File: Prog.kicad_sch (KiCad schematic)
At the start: 23 parts, among them J2 JTAG, J3 microUSB, Q1 MMBT3904, Q2 MMBT3904, U12 CH340G, U7 74AHCT573PW, Y1 12M

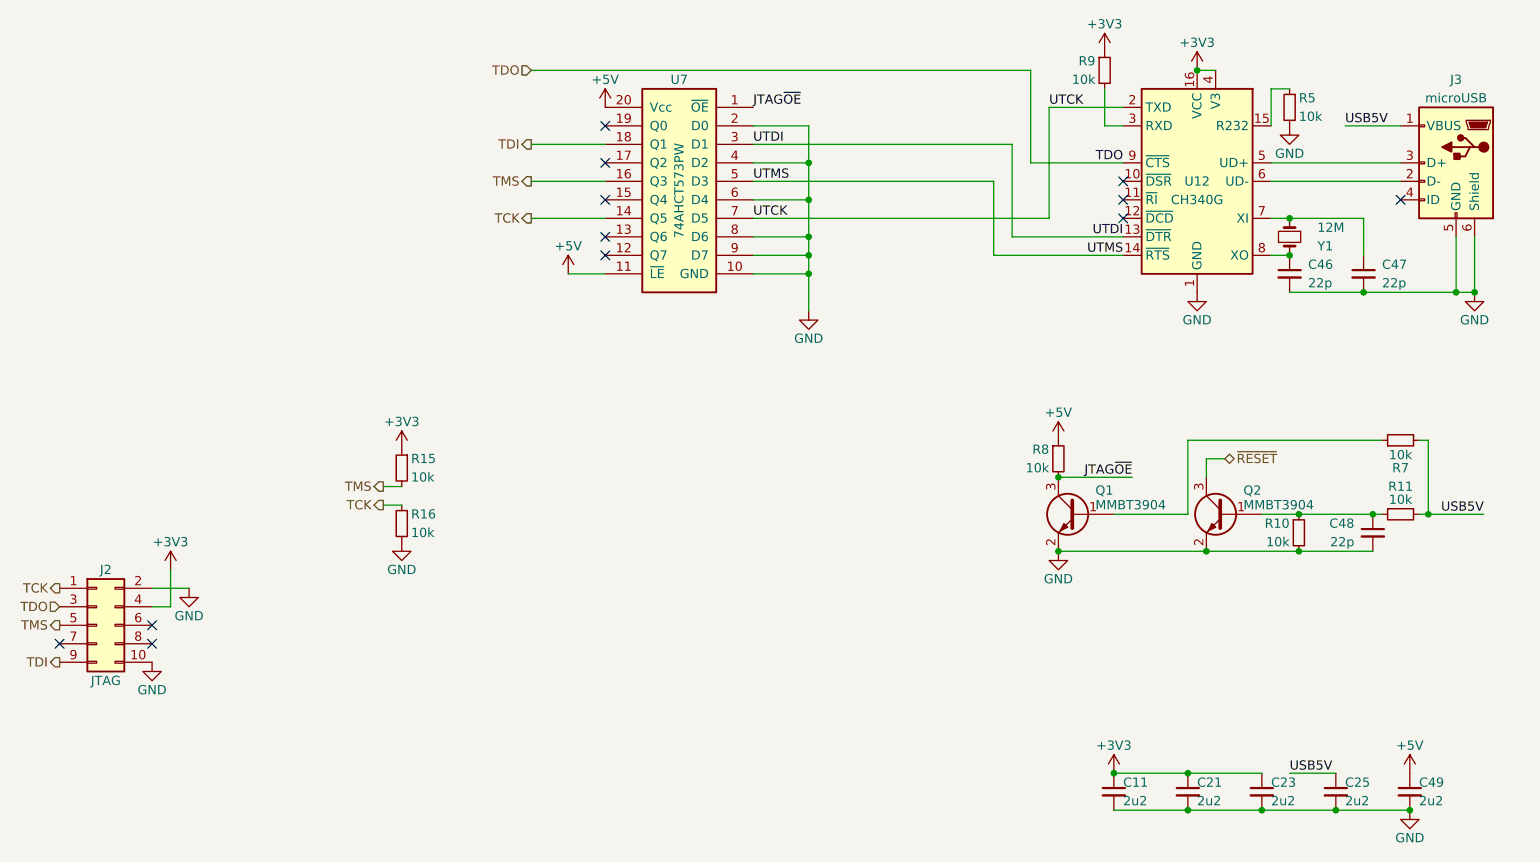
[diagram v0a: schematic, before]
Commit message: idk
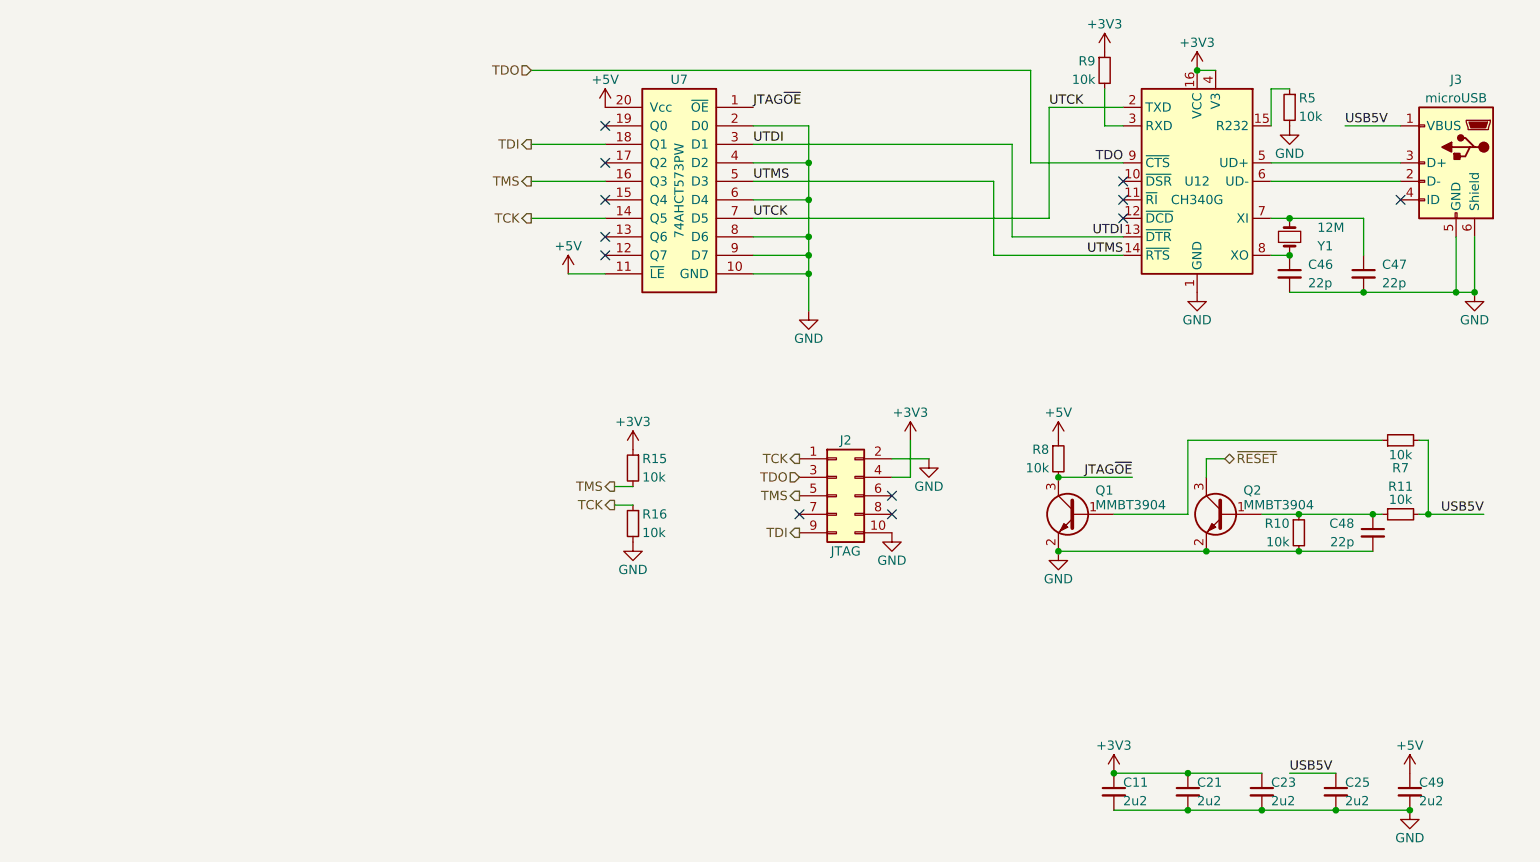
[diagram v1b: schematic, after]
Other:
- moved on the sheet: J2, R15, R16

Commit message: Toward final "A"
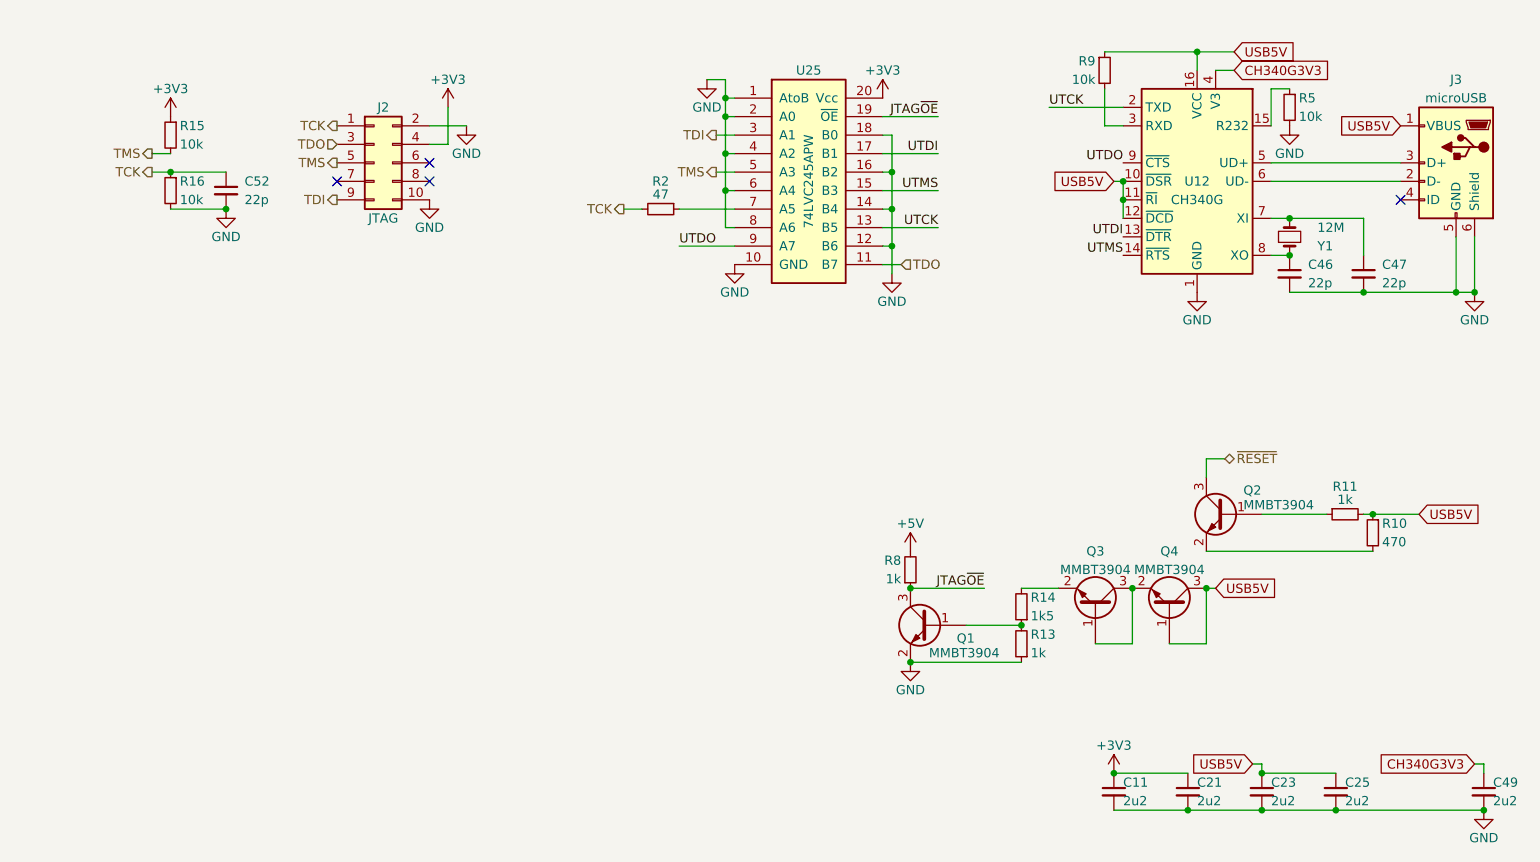
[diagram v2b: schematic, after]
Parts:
- removed C48: 22p, stdpads:C_0603, symbol Device:C_Small
- removed R7: 10k, stdpads:R_0603, symbol Device:R_Small
- removed U7: 74AHCT573PW, stdpads:TSSOP-20_4.4x6.5mm_P0.65mm, symbol GW_Logic:74573
- added C52: 22p, stdpads:C_0603, symbol Device:C_Small
- added Q3, Q4: MMBT3904, stdpads:SOT-23, symbol Transistor_BJT:MMBT3904
- added R13: 1k, stdpads:R_0603, symbol Device:R_Small
- added R14: 1k5, stdpads:R_0603, symbol Device:R_Small
- added R2: 47, stdpads:R_0603, symbol Device:R_Small
- added U25: 74LVC245APW, stdpads:TSSOP-20_4.4x6.5mm_P0.65mm, symbol GW_Logic:74245
- R10: value 10k -> 470; footprint stdpads:R_0603 -> stdpads:R_0805; LCSC Part C25804 -> (none)
- R11, R8: value 10k -> 1k; LCSC Part C25804 -> (none)
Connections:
- net +3V3: now also U25.20 (Vcc); no longer C23.1, R9.1, U12.16 (VCC), U12.4 (V3)
- net +5V: now also R8.2; no longer C49.1, R8.1
- net GND: now also C52.2, R13.1, U25.1 (AtoB), U25.10 (GND), U25.12 (B6), U25.14 (B4), U25.16 (B2), U25.18 (B0), U25.2 (A0), U25.4 (A2), U25.6 (A4), U25.8 (A6); no longer Q2.2 (E), R10.2
- net JTAG~{OE}: now also R8.1, U25.19 (~{OE}); no longer R8.2
- net TCK: now also C52.1, R2.2
- net TDI: now also U25.3 (A1)
- net TDO: now also U25.11 (B7); no longer U12.9 (~{CTS})
- net TMS: now also U25.5 (A3)
- net USB5V: now also C23.1, R10.1, R9.1, U12.10 (~{DSR}), U12.11 (~{RI}), U12.12 (~{DCD}), U12.16 (VCC), Q4.1 (B), Q4.3 (C)
- net UTCK: now also U25.13 (B5)
- net UTDI: now also U25.17 (B1)
- net UTMS: now also U25.15 (B3)
- net at Q2.1 (B), R11.1: no longer R10.1
- net at Q1.1 (B): now also R13.2, R14.1
- new net: Q2.2 (E), R10.2
- new net: R2.1, U25.7 (A5)
- new net: Q3.2 (E), R14.2
- new net: Q3.1 (B), Q3.3 (C), Q4.2 (E)
- new net CH340G3V3: C49.1, U12.4 (V3)
- new net UTDO: U12.9 (~{CTS}), U25.9 (A7)
- no-connect marks 12 -> 4
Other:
- moved on the sheet: C49, J2, Q1, R10, R15, R16

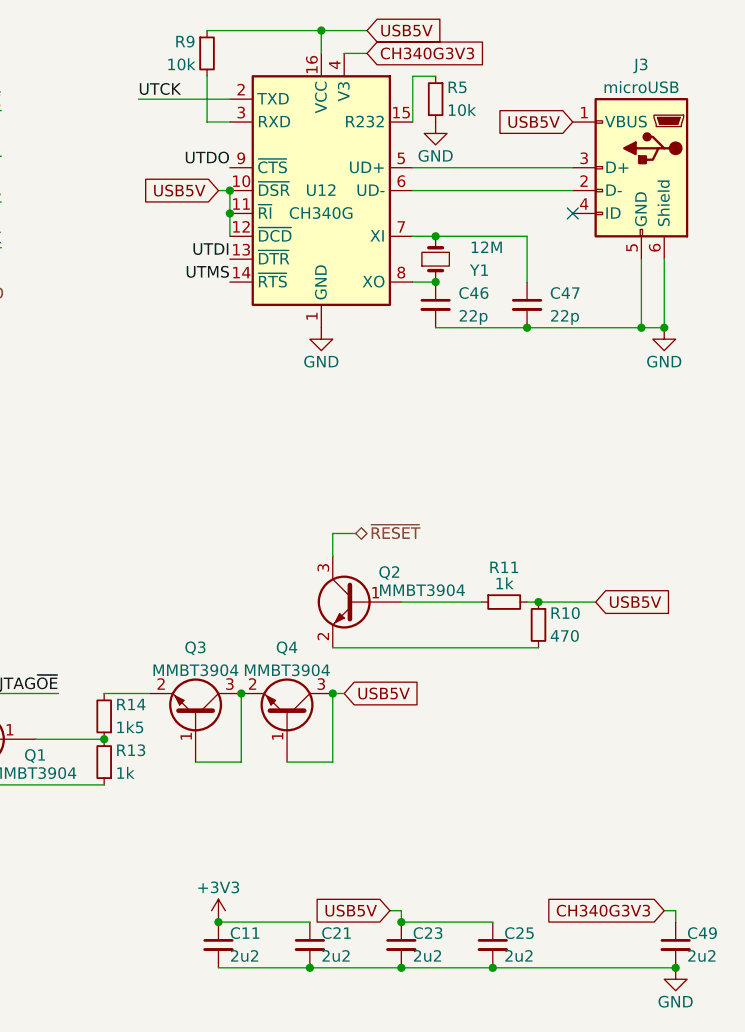
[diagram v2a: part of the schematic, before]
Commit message: idk
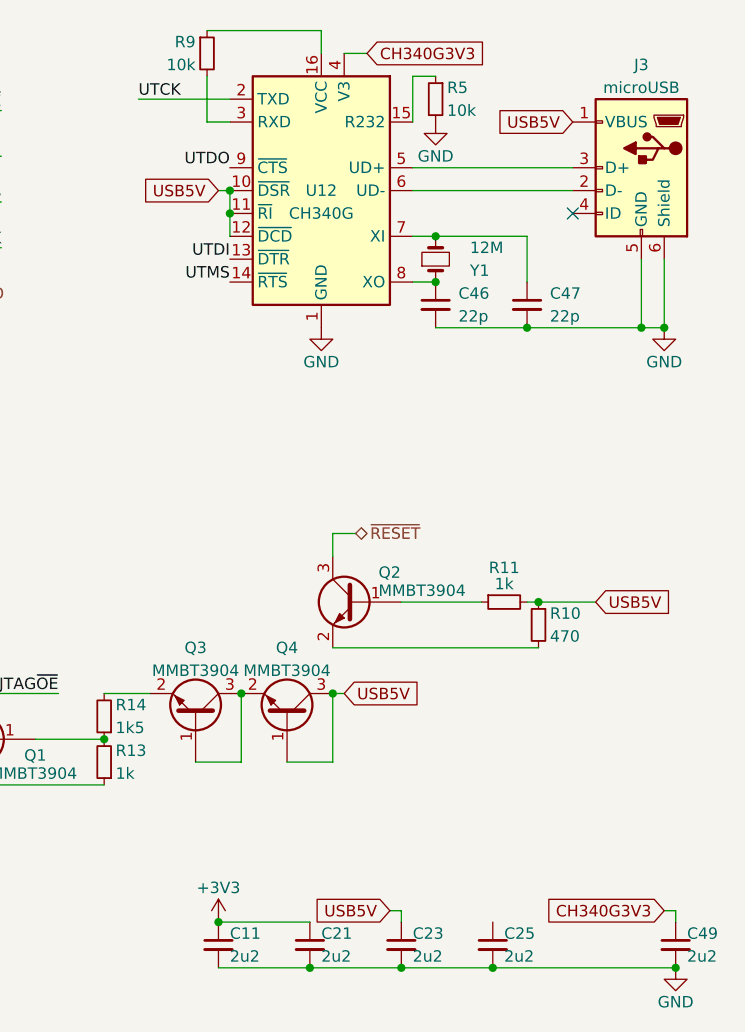
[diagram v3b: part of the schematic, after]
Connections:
- net USB5V: no longer C25.1, R9.1, U12.16 (VCC)
- new net: R9.1, U12.16 (VCC)
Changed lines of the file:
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@@
   (junction (at 156.21 48.26) (diameter 0) (color 0 0 0 0)
   )
-  (junction (at 220.98 41.91) (diameter 0) (color 0 0 0 0)
-  )
   (junction (at 179.07 63.5) (diameter 0) (color 0 0 0 0)
   )
@@
   )
   (junction (at 260.35 146.05) (diameter 0) (color 0 0 0 0)
-  )
-  (junction (at 229.87 140.97) (diameter 0) (color 0 0 0 0)
   )
   (junction (at 219.71 146.05) (diameter 0) (color 0 0 0 0)
@@
     (stroke (width 0) (type default))
   )
-  (wire (pts (xy 229.87 140.97) (xy 240.03 140.97))
-    (stroke (width 0) (type default))
-  )
   (wire (pts (xy 208.28 46.99) (xy 208.28 52.07))
     (stroke (width 0) (type default))
@@
   )
   (wire (pts (xy 224.79 97.79) (xy 222.25 97.79))
-    (stroke (width 0) (type default))
-  )
-  (wire (pts (xy 220.98 41.91) (xy 226.06 41.91))
     (stroke (width 0) (type default))
   )
@@
     )
   )
-  (global_label "USB5V" (shape input) (at 226.06 41.91 0) (fields_autoplaced)
-    (effects (font (size 1.27 1.27)) (justify left))
-    (property "Intersheetrefs" "${INTERSHEET_REFS}" (at 234.4197 41.91 0)
-      (effects (font (size 1.27 1.27)) (justify left) hide)
-    )
-  )

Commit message: Revert "idk"
This reverts commit aa30aa8a559ae1d3e965923a55380a6d00f93ea4.
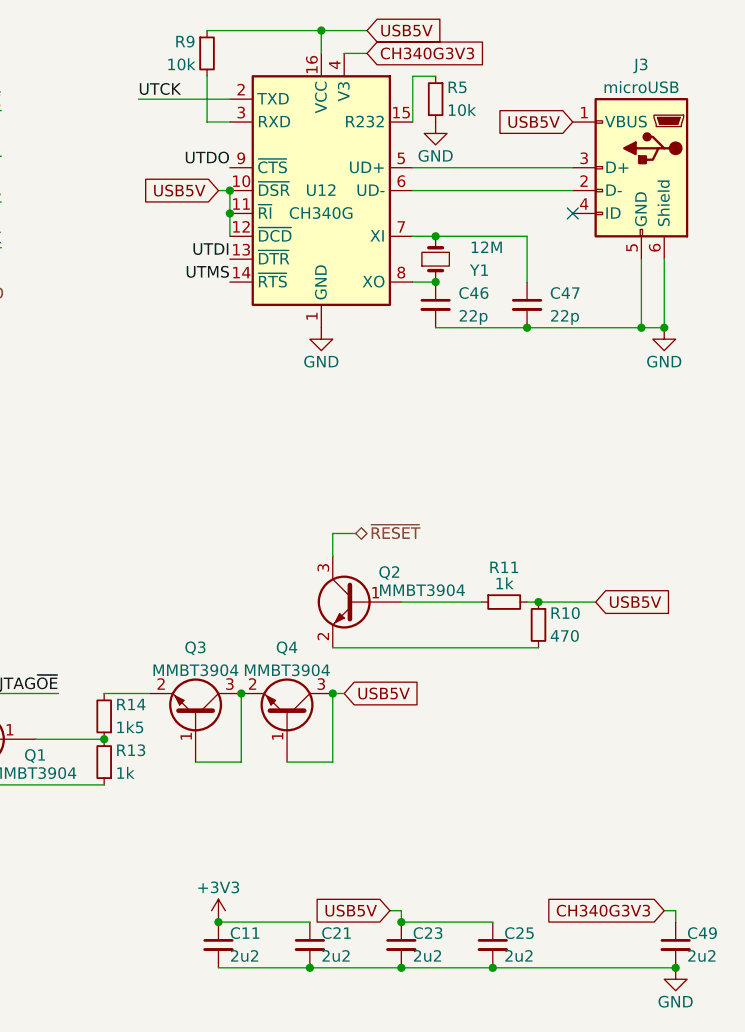
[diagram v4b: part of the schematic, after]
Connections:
- net USB5V: now also C25.1, R9.1, U12.16 (VCC)
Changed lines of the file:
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@@
   (junction (at 156.21 48.26) (diameter 0) (color 0 0 0 0)
   )
+  (junction (at 220.98 41.91) (diameter 0) (color 0 0 0 0)
+  )
   (junction (at 179.07 63.5) (diameter 0) (color 0 0 0 0)
   )
@@
   )
   (junction (at 260.35 146.05) (diameter 0) (color 0 0 0 0)
+  )
+  (junction (at 229.87 140.97) (diameter 0) (color 0 0 0 0)
   )
   (junction (at 219.71 146.05) (diameter 0) (color 0 0 0 0)
@@
     (stroke (width 0) (type default))
   )
+  (wire (pts (xy 229.87 140.97) (xy 240.03 140.97))
+    (stroke (width 0) (type default))
+  )
   (wire (pts (xy 208.28 46.99) (xy 208.28 52.07))
     (stroke (width 0) (type default))
@@
   )
   (wire (pts (xy 224.79 97.79) (xy 222.25 97.79))
+    (stroke (width 0) (type default))
+  )
+  (wire (pts (xy 220.98 41.91) (xy 226.06 41.91))
     (stroke (width 0) (type default))
   )
@@
     )
   )
+  (global_label "USB5V" (shape input) (at 226.06 41.91 0) (fields_autoplaced)
+    (effects (font (size 1.27 1.27)) (justify left))
+    (property "Intersheetrefs" "${INTERSHEET_REFS}" (at 234.4197 41.91 0)
+      (effects (font (size 1.27 1.27)) (justify left) hide)
+    )
+  )
